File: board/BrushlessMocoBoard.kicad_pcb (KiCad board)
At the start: 4 copper layers, 115 parts, among them SW1 SW_Push, SW2 SW_Push, U1 STSPIN32G4TR, U2 SN65HVD232

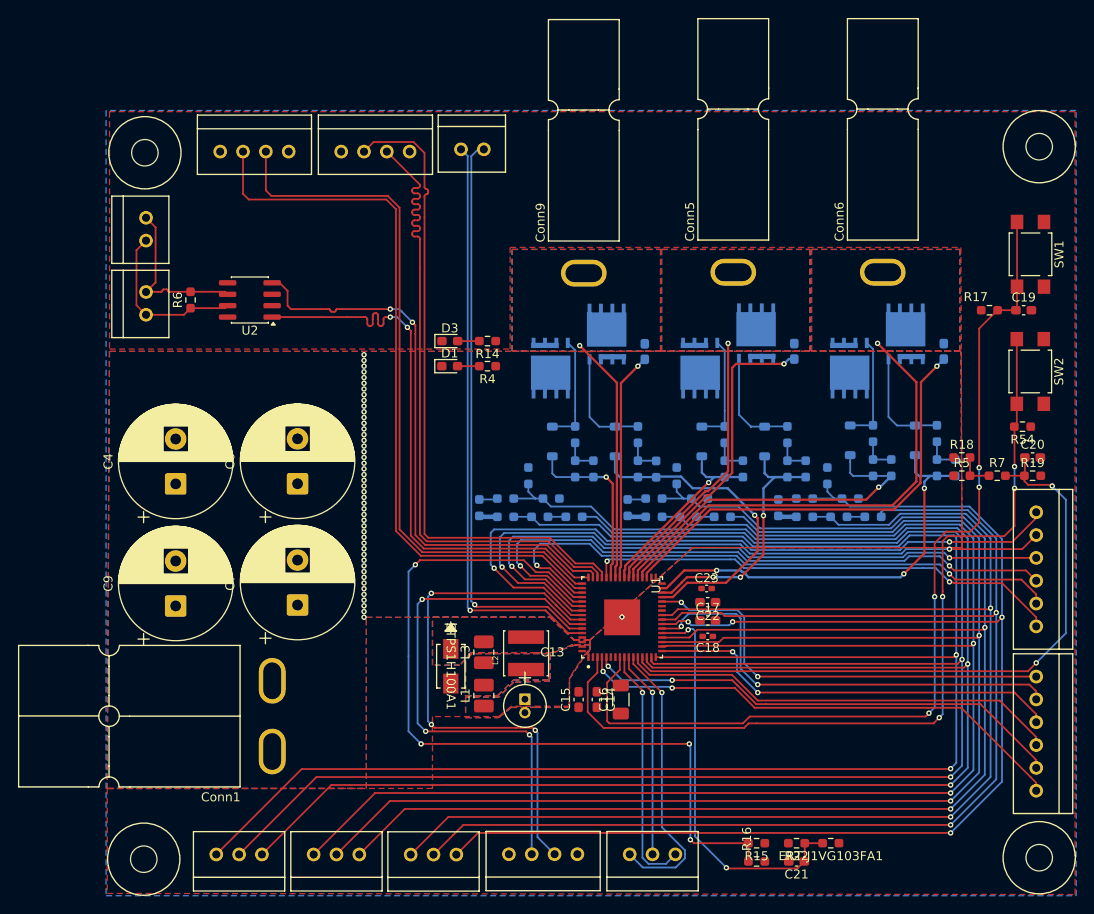
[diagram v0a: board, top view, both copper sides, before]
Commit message: Tentatively finished rev1.
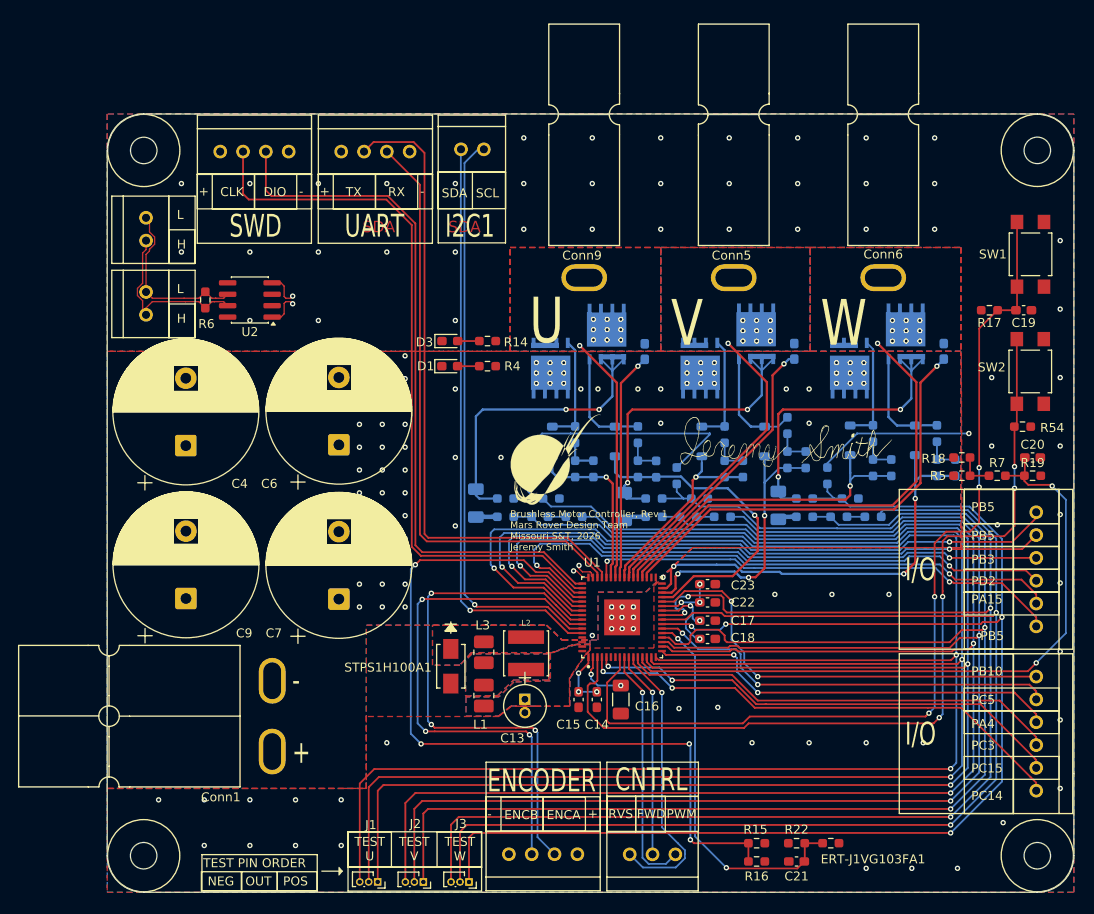
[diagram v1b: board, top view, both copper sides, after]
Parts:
- removed Conn14, Conn15, Conn16: Molex_SL_03, MRDT_Connectors:MOLEX_SL_03_Vertical
- added ?: , clipboard:e9d430d6-ea22-4c50-aad5-93117c9e5b7d, F.Cu at (105.5, 73.1)
- added G***: LOGO, MRDT_Silkscreens:0_MRDT_Logo_10mm, F.Cu at (79.8, 79.0)
- added J1: Conn_01x03, Connector_PinSocket_1.00mm:PinSocket_1x03_P1.00mm_Vertical, F.Cu at (59.9, 126.0)
- added J2: Conn_01x03, Connector_PinSocket_1.00mm:PinSocket_1x03_P1.00mm_Vertical, F.Cu at (65.0, 126.0)
- added J3: Conn_01x03, Connector_PinSocket_1.00mm:PinSocket_1x03_P1.00mm_Vertical, F.Cu at (70.1, 126.0)
- C18, C23: footprint Capacitor_SMD:C_0402_1005Metric_Pad0.74x0.62mm_HandSolder -> Capacitor_SMD:C_0603_1608Metric_Pad1.08x0.95mm_HandSolder
- C4, C6, C7, C9: footprint Capacitor_THT:CP_Radial_D12.5mm_P5.00mm -> Capacitor_THT:CP_Radial_D16.0mm_P7.50mm
- R3, R43, R50: footprint Resistor_SMD:R_0603_1608Metric_Pad0.98x0.95mm_HandSolder -> Resistor_SMD:R_1206_3216Metric_Pad1.30x1.75mm_HandSolder
- moved C6 6.32 mm to (55.6, 77.3)
- moved C7 4.65 mm to (55.6, 94.5)
- moved C4 4.41 mm to (38.6, 77.4)
- moved R6 1.64 mm to (40.8, 61.2)
- moved C9 1.41 mm to (38.6, 94.4)
- moved R10 1.02 mm to (105.5, 79.0)
- moved R11 1.02 mm to (107.6, 79.0)
- moved R13 1.02 mm to (105.5, 75.2)
- moved R3 0.64 mm to (70.9, 83.8)
- moved Conn6 0.61 mm to (116.3, 59.0)
- moved Conn5 0.61 mm to (99.7, 59.0)
- moved Conn9 0.50 mm to (83.0, 59.0)
- moved C23 0.49 mm to (96.6, 92.8)
- moved H2 0.46 mm to (133.3, 44.6)
- moved R43 0.40 mm to (87.4, 84.2)
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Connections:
- net /Interfaces/CAN_RX renamed /MCU/CANX-
- net /Interfaces/CAN_TX renamed /MCU/CANX+
- net CANH renamed CAN+
- net CANL renamed CAN-
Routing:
- net +3.3V: track 0.00 -> 74.8 mm, vias 0 -> 81
- net Vs_V_High: track 2.05 -> 35.2 mm, vias 0 -> 2
- net Vs_U_High: track 2.05 -> 35.1 mm, vias 0 -> 2
- net Vs_W_High: track 2.05 -> 34.7 mm, vias 0 -> 2
- net /Half-Bridges & Current Sensing/OPN_U: track 196.5 -> 188.5 mm
- net /Half-Bridges & Current Sensing/OPO_U: track 189.5 -> 182.5 mm
- net /Interfaces/UART_RX: track 72.5 -> 66.2 mm
- net /Half-Bridges & Current Sensing/OPP_U: track 200.1 -> 194.4 mm
- net /Half-Bridges & Current Sensing/OPN_W: track 153.3 -> 158.8 mm, vias 2 -> 4
- net /Interfaces/I/O_PC5: track 50.4 -> 46.3 mm
- net /Half-Bridges & Current Sensing/OUT_V: track 30.8 -> 34.2 mm, vias 1 -> 10
- net /Half-Bridges & Current Sensing/BOOT_V: track 35.4 -> 32.1 mm
- net /Half-Bridges & Current Sensing/OPN_V: track 174.8 -> 171.6 mm
- net /Half-Bridges & Current Sensing/GHS_W: track 40.0 -> 37.1 mm
- net /Half-Bridges & Current Sensing/OPP_W: track 154.5 -> 157.4 mm
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- added copper zone on In1.Cu, net +3.3V
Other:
- board outline added: 107.6 x 86.6 mm
- board text added: "+"
- board text added: "-"
- board text added: "Brushless Motor Controller, Rev 1 Mars Rover Design Team Missouri S&T, 2026 Jeremy Smith"
- board text added: "CLK"
- board text added: "CNTRL"
- board text added: "DIO"
- board text added: "ENCA"
- board text added: "ENCB"
- board text added: "ENCODER"
- board text added: "FWD"
- board text added: "H"
- board text added: "I/O"
- board text added: "I2C1"
- board text added: "L"
- board text added: "NEG"
- board text added: "OUT"
- board text added: "PA15"
- board text added: "PA4"
- board text added: "PB10"
- board text added: "PB3"
- board text added: "PB5"
- board text added: "PC14"
- board text added: "PC15"
- board text added: "PC3"
- board text added: "PC5"
- board text added: "PD2"
- board text added: "POS"
- board text added: "PWM"
- board text added: "RVS"
- board text added: "RX"
- board text added: "SCL"
- board text added: "SDA"
- board text added: "SWD"
- board text added: "TEST PIN ORDER"
- board text added: "TEST U"
- board text added: "TEST V"
- board text added: "TEST W"
- board text added: "TX"
- board text added: "U"
- board text added: "UART"
- board text added: "V"
- board text added: "W"
